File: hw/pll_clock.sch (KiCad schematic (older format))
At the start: 22 parts, among them J7 BNC, J8 BNC, U7 5P49V5925, Y1 25MHz

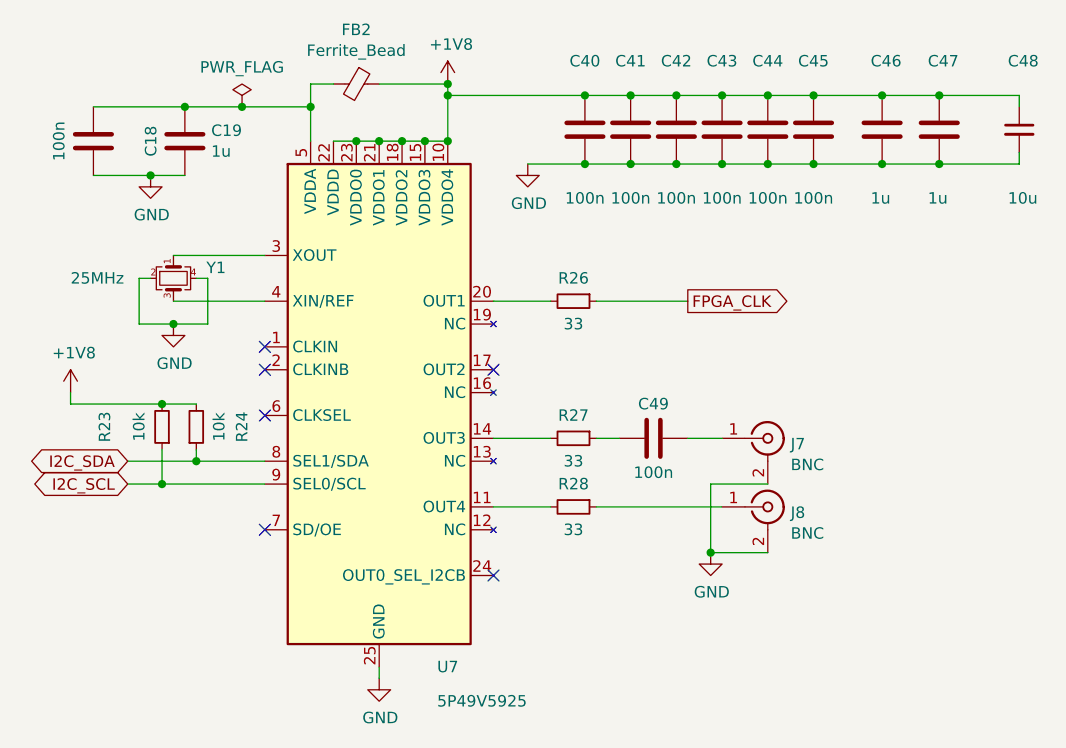
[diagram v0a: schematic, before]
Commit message: several updates...
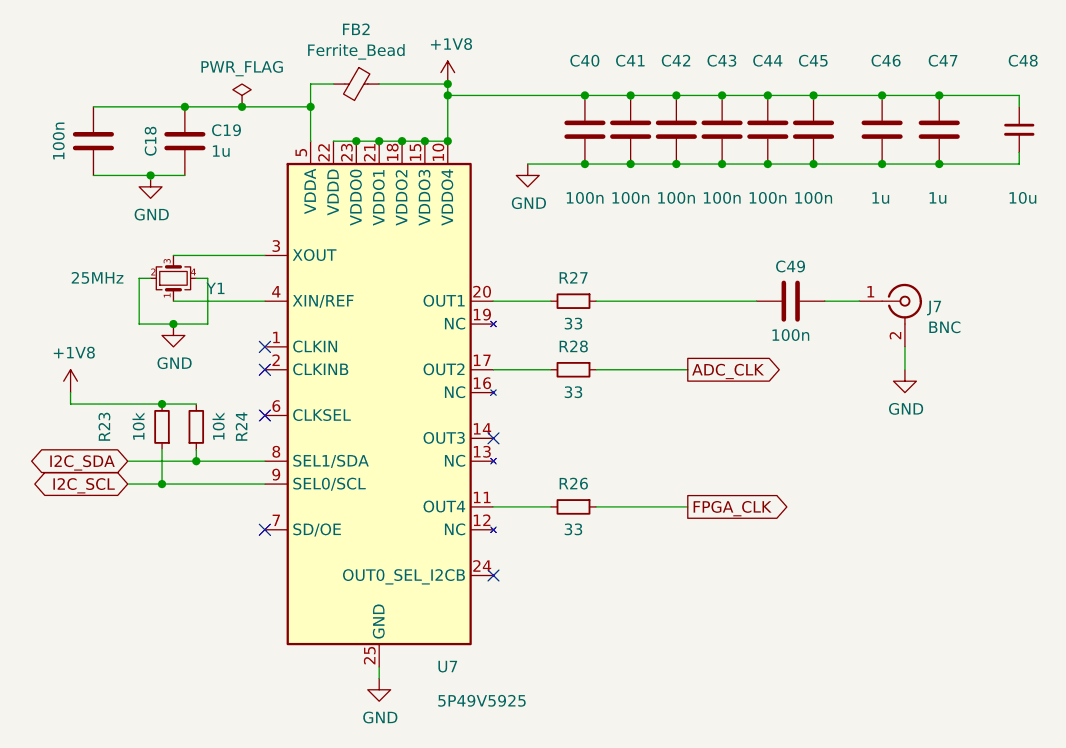
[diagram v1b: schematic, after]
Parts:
- removed J8: BNC, proj_footprints:BNC_Molex_0731713150, symbol Connector:Conn_Coaxial
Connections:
- net ADC_CLK: now reaches R28.1
- net at Y1.1: now also U7.4 (XIN/REF); no longer U7.3 (XOUT)
- net at Y1.3: now also U7.3 (XOUT); no longer U7.4 (XIN/REF)
- net at R27.2: now also U7.20 (OUT1); no longer U7.14 (OUT3)
- net at R28.2: now also U7.17 (OUT2); no longer U7.11 (OUT4)
- net at R26.2: now also U7.11 (OUT4); no longer U7.20 (OUT1)
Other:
- moved on the sheet: C49, J7, R26, R27, R28
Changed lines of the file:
@@
 $Descr A4 11693 8268
 encoding utf-8
-Sheet 4 4
+Sheet 4 5
 Title ""
 Date ""
@@
 NoConn ~ 5100 3900
 NoConn ~ 5100 3400
-NoConn ~ 6100 3200
 NoConn ~ 5100 3100
 NoConn ~ 5100 3200
@@
 F 5 "Abracon" V 4700 2800 50  0001 C CNN "Manufacturer"
 	1    4700 2800
-	0    1    1    0
+	0    1    -1   0
 $EndComp
 Wire Wire Line
@@
 Wire Wire Line
 	4500 3700 4650 3700
-Text GLabel 6950 2900 2    50   Output ~ 0
+Text GLabel 6950 3800 2    50   Output ~ 0
 FPGA_CLK
 Wire Wire Line
-	6100 2900 6350 2900
+	6100 3800 6350 3800
 $Comp
 L Device:R_Small R?
@@
 L Device:R_Small R?
 U 1 1 60D6AA6F
-P 6450 2900
+P 6450 3800
 AR Path="/60AABC24/60D6AA6F" Ref="R?"  Part="1"
 AR Path="/60B16D71/60D6AA6F" Ref="R26"  Part="1"
-F 0 "R26" V 6350 2900 50  0000 C CNN
-F 1 "33" V 6550 2900 50  0000 C CNN
-F 2 "Resistor_SMD:R_0603_1608Metric" H 6450 2900 50  0001 C CNN
-F 3 "~" H 6450 2900 50  0001 C CNN
-F 4 " RC0603FR-0733RL " V 6450 2900 50  0001 C CNN "Part"
-F 5 "Yageo" V 6450 2900 50  0001 C CNN "Manufacturer"
-	1    6450 2900
+F 0 "R26" V 6350 3800 50  0000 C CNN
+F 1 "33" V 6550 3800 50  0000 C CNN
+F 2 "Resistor_SMD:R_0603_1608Metric" H 6450 3800 50  0001 C CNN
+F 3 "~" H 6450 3800 50  0001 C CNN
+F 4 " RC0603FR-0733RL " V 6450 3800 50  0001 C CNN "Part"
+F 5 "Yageo" V 6450 3800 50  0001 C CNN "Manufacturer"
+	1    6450 3800
 	0    1    1    0
 $EndComp
 Wire Wire Line
-	6550 2900 6950 2900
+	6550 3800 6950 3800
 $Comp
 L fmc:100nF_603 C?
@@
 	5000 2050 5300 2050
 Wire Wire Line
-	6100 3500 6350 3500
-Wire Wire Line
-	6100 3800 6350 3800
-$Comp
-L Connector:Conn_Coaxial J8
-U 1 1 6092C0EF
-P 7300 3800
-F 0 "J8" H 7400 3775 50  0000 L CNN
-F 1 "BNC" H 7400 3684 50  0000 L CNN
-F 2 "proj_footprints:BNC_Molex_0731713150" H 7300 3800 50  0001 C CNN
-F 3 " ~" H 7300 3800 50  0001 C CNN
-F 4 "0731713150" H 7300 3800 50  0001 C CNN "Part"
-F 5 "Molex" H 7300 3800 50  0001 C CNN "Manufacturer"
-	1    7300 3800
-	1    0    0    -1
-$EndComp
-Wire Wire Line
-	6550 3800 7100 3800
-Wire Wire Line
-	7300 3700 7050 3700
-Wire Wire Line
-	7050 3700 7050 4000
-Wire Wire Line
-	7050 4000 7300 4000
+	6100 2900 6350 2900
+Wire Wire Line
+	6100 3200 6350 3200
 $Comp
 L power:GND #PWR?
 U 1 1 6092DB98
-P 7050 4000
+P 7900 3200
 AR Path="/6086F2E3/6092DB98" Ref="#PWR?"  Part="1"
 AR Path="/60AABC24/6092DB98" Ref="#PWR?"  Part="1"
 AR Path="/60B16D71/6092DB98" Ref="#PWR?"  Part="1"
-F 0 "#PWR?" H 7050 3750 50  0001 C CNN
-F 1 "GND" H 7055 3827 50  0000 C CNN
-F 2 "" H 7050 4000 50  0001 C CNN
-F 3 "" H 7050 4000 50  0001 C CNN
-	1    7050 4000
-	1    0    0    -1
-$EndComp
-Connection ~ 7050 4000
+F 0 "#PWR?" H 7900 2950 50  0001 C CNN
+F 1 "GND" H 7905 3027 50  0000 C CNN
+F 2 "" H 7900 3200 50  0001 C CNN
+F 3 "" H 7900 3200 50  0001 C CNN
+	1    7900 3200
+	1    0    0    -1
+$EndComp
 $Comp
 L fmc:100nF_603 C?
@@
 L Device:R_Small R?
 U 1 1 60C371EA
-P 6450 3500
+P 6450 2900
 AR Path="/60AABC24/60C371EA" Ref="R?"  Part="1"
 AR Path="/60B16D71/60C371EA" Ref="R27"  Part="1"
-F 0 "R27" V 6350 3500 50  0000 C CNN
-F 1 "33" V 6550 3500 50  0000 C CNN
-F 2 "Resistor_SMD:R_0603_1608Metric" H 6450 3500 50  0001 C CNN
-F 3 "~" H 6450 3500 50  0001 C CNN
-F 4 " RC0603FR-0733RL " V 6450 3500 50  0001 C CNN "Part"
-F 5 "Yageo" V 6450 3500 50  0001 C CNN "Manufacturer"
-	1    6450 3500
+F 0 "R27" V 6350 2900 50  0000 C CNN
+F 1 "33" V 6550 2900 50  0000 C CNN
+F 2 "Resistor_SMD:R_0603_1608Metric" H 6450 2900 50  0001 C CNN
+F 3 "~" H 6450 2900 50  0001 C CNN
+F 4 " RC0603FR-0733RL " V 6450 2900 50  0001 C CNN "Part"
+F 5 "Yageo" V 6450 2900 50  0001 C CNN "Manufacturer"
+	1    6450 2900
 	0    1    1    0
 $EndComp
@@
 L Device:R_Small R?
 U 1 1 60C375F6
-P 6450 3800
+P 6450 3200
 AR Path="/60AABC24/60C375F6" Ref="R?"  Part="1"
 AR Path="/60B16D71/60C375F6" Ref="R28"  Part="1"
-F 0 "R28" V 6350 3800 50  0000 C CNN
-F 1 "33" V 6550 3800 50  0000 C CNN
-F 2 "Resistor_SMD:R_0603_1608Metric" H 6450 3800 50  0001 C CNN
-F 3 "~" H 6450 3800 50  0001 C CNN
-F 4 " RC0603FR-0733RL " V 6450 3800 50  0001 C CNN "Part"
-F 5 "Yageo" V 6450 3800 50  0001 C CNN "Manufacturer"
-	1    6450 3800
+F 0 "R28" V 6350 3200 50  0000 C CNN
+F 1 "33" V 6550 3200 50  0000 C CNN
+F 2 "Resistor_SMD:R_0603_1608Metric" H 6450 3200 50  0001 C CNN
+F 3 "~" H 6450 3200 50  0001 C CNN
+F 4 " RC0603FR-0733RL " V 6450 3200 50  0001 C CNN "Part"
+F 5 "Yageo" V 6450 3200 50  0001 C CNN "Manufacturer"
+	1    6450 3200
 	0    1    1    0
 $EndComp
@@
 L Connector:Conn_Coaxial J7
 U 1 1 60C731B4
-P 7300 3500
-F 0 "J7" H 7400 3475 50  0000 L CNN
-F 1 "BNC" H 7400 3384 50  0000 L CNN
-F 2 "proj_footprints:BNC_Molex_0731713150" H 7300 3500 50  0001 C CNN
-F 3 " ~" H 7300 3500 50  0001 C CNN
-F 4 "0731713150" H 7300 3500 50  0001 C CNN "Part"
-F 5 "Molex" H 7300 3500 50  0001 C CNN "Manufacturer"
-	1    7300 3500
+P 7900 2900
+F 0 "J7" H 8000 2875 50  0000 L CNN
+F 1 "BNC" H 8000 2784 50  0000 L CNN
+F 2 "proj_footprints:BNC_Molex_0731713150" H 7900 2900 50  0001 C CNN
+F 3 " ~" H 7900 2900 50  0001 C CNN
+F 4 "0731713150" H 7900 2900 50  0001 C CNN "Part"
+F 5 "Molex" H 7900 2900 50  0001 C CNN "Manufacturer"
+	1    7900 2900
 	1    0    0    -1
 $EndComp
@@
 L fmc:100nF_603 C?
 U 1 1 60B85B4A
-P 6800 3500
+P 7400 2900
 AR Path="/6086F2E3/60B85B4A" Ref="C?"  Part="1"
 AR Path="/60B16D71/60B85B4A" Ref="C49"  Part="1"
-F 0 "C49" V 6950 3500 50  0000 C CNN
-F 1 "100n" V 6650 3500 50  0000 C CNN
-F 2 "Capacitor_SMD:C_0603_1608Metric" H 6838 3350 50  0001 C CNN
-F 3 "~" H 6800 3500 50  0001 C CNN
-F 4 "GCJ188R71E104KA12D" H 6925 3700 50  0001 C CNN "Part"
-F 5 "Murata" H 7025 3800 50  0001 C CNN "Manufacturer"
-	1    6800 3500
+F 0 "C49" V 7550 2900 50  0000 C CNN
+F 1 "100n" V 7250 2900 50  0000 C CNN
+F 2 "Capacitor_SMD:C_0603_1608Metric" H 7438 2750 50  0001 C CNN
+F 3 "~" H 7400 2900 50  0001 C CNN
+F 4 "GCJ188R71E104KA12D" H 7525 3100 50  0001 C CNN "Part"
+F 5 "Murata" H 7625 3200 50  0001 C CNN "Manufacturer"
+	1    7400 2900
 	0    -1   -1   0
 $EndComp
 Wire Wire Line
-	6950 3500 7100 3500
-Wire Wire Line
-	6550 3500 6650 3500
+	7550 2900 7700 2900
 Wire Wire Line
 	5500 2200 5600 2200
@@
 Wire Wire Line
 	5800 2200 5900 2200
+NoConn ~ 6100 3500
+Text GLabel 6950 3200 2    50   Output ~ 0
+ADC_CLK
+Wire Wire Line
+	6550 3200 6950 3200
+Wire Wire Line
+	6550 2900 7250 2900
+Wire Wire Line
+	7900 3100 7900 3200
 $EndSCHEMATC
